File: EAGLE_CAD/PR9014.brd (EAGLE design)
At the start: 68.1 x 70.2 mm, 69 parts, among them J1 M3_SCREW_POST, SW1 C&K_PTS645

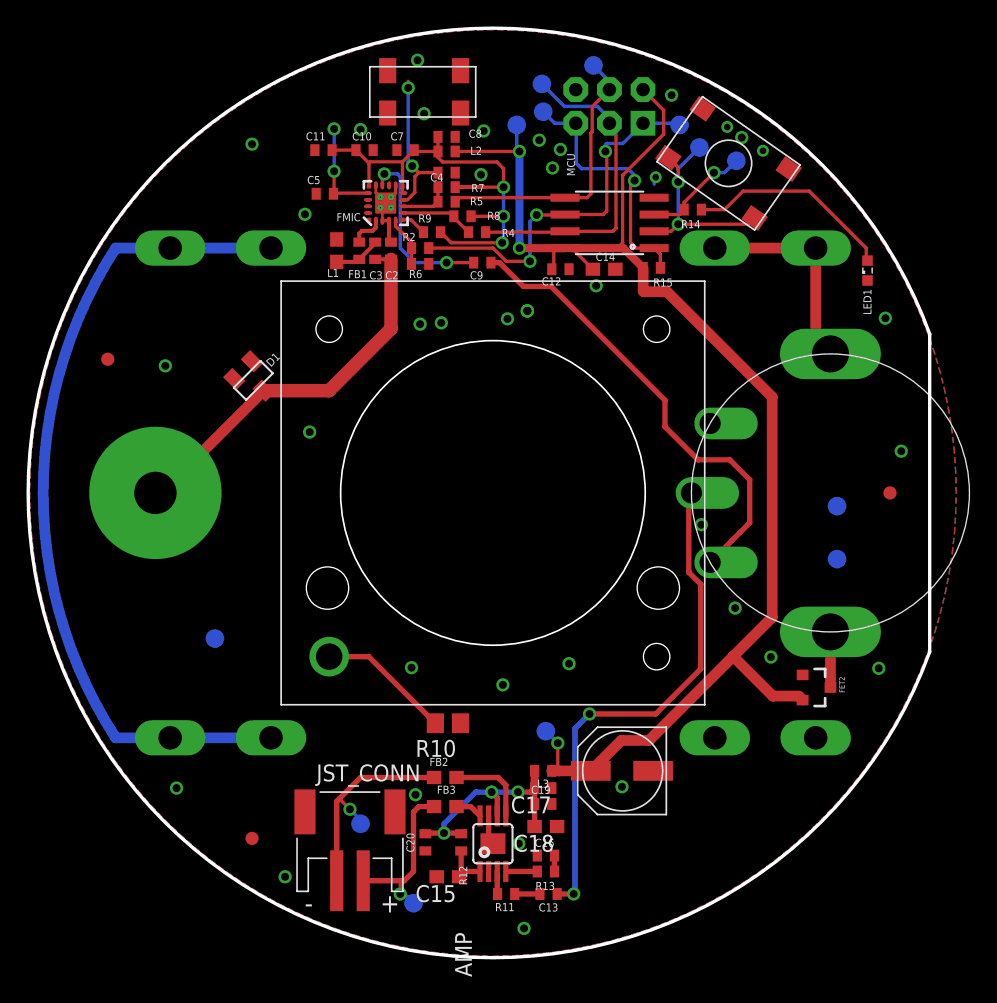
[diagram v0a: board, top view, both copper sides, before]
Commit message: bunch of routing stuff
and made the test points larger

pretty close to being released for this round
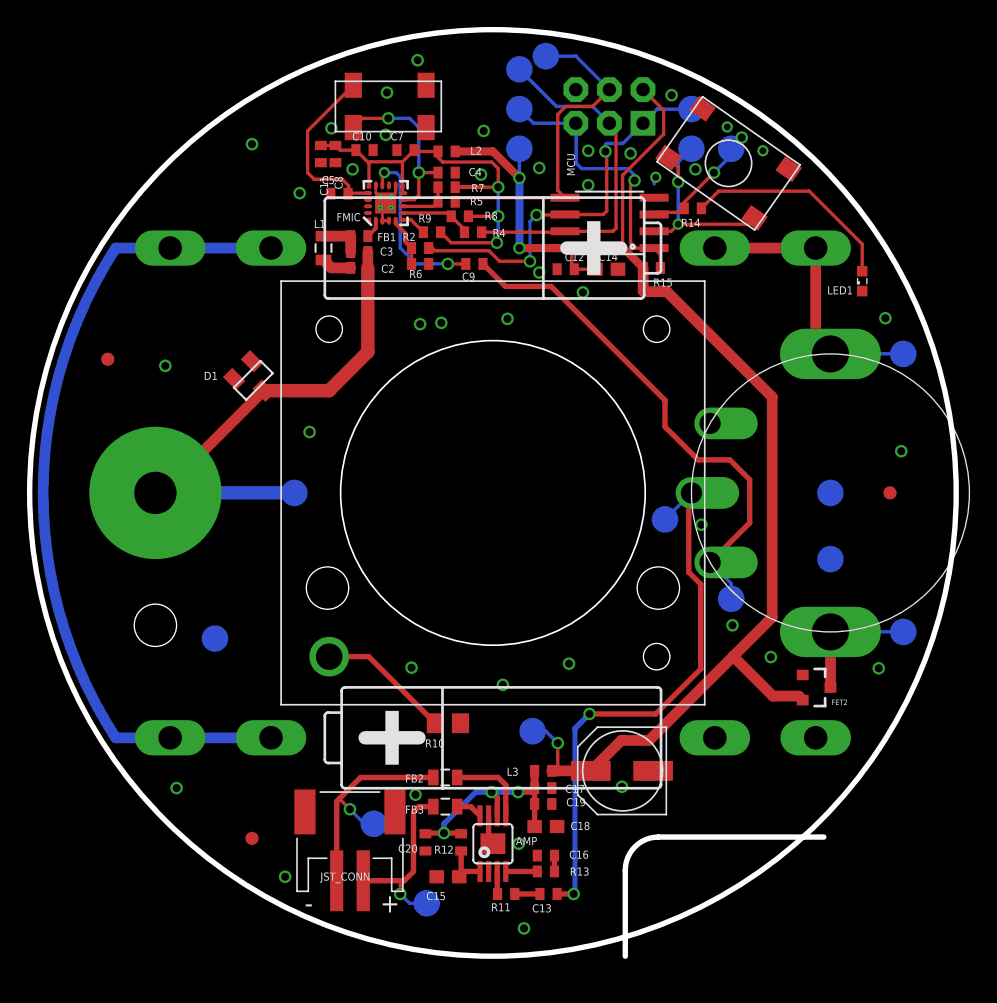
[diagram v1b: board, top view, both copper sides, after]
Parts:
- added TP14, TP15, TP16, TP17, TP18: TPTP20R, testpad:TP20R
- FB2, FB3, L1: device SparkFun-Passives:0603 -> SparkFun-Passives:0805
- TP1, TP10, TP11, TP12, TP13, TP2, TP3, TP4, TP5, TP6, TP7, TP8, TP9: value TPTP14R -> TPTP20R; device testpad:TP14R -> testpad:TP20R
- moved C8 8.50 mm to (23.1, 60.6), turned to 270 degrees
- moved TP13 3.67 mm to (39.0, 68.0)
- moved U$6 2.82 mm to (27.2, 64.2)
- moved C2 2.73 mm to (24.9, 52.0), turned to 180 degrees
- moved TP11 2.02 mm to (37.0, 67.0)
- moved TP12 1.81 mm to (37.0, 64.0)
- moved TP5 1.81 mm to (37.0, 61.0)
- moved TP10 1.50 mm to (50.0, 64.0)
- moved C3 1.20 mm to (24.9, 53.2), turned to 180 degrees
- moved TP2 1.12 mm to (60.5, 35.0)
- moved FB1 1.10 mm to (24.9, 54.4), turned to 0 degrees
- moved C5 1.10 mm to (23.4, 57.6)
- moved L1 1.02 mm to (22.2, 53.5), turned to 270 degrees
- moved TP4 1.00 mm to (38.0, 17.0)
- moved TP6 1.00 mm to (26.0, 10.0)
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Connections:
- removed net N$14: C2.1, C3.1, D1.3, J1.P$1
- removed net N$15: JP5.POS, JP5.POS@2, R1.SW_OUT
- removed net N$2: C5.1, FMIC.17, U$6.P$1
- removed net N$34: FET2.3, R1.SW_IN
- new net ANT: C2.1, C3.1, D1.3, J1.P$1, TP18.TP
- new net N$10: C5.1, FMIC.17, U$6.P$4
- new net SW_IN: FET2.3, R1.SW_IN, TP14.TP
- new net SW_OUT: JP5.POS, JP5.POS@2, R1.SW_OUT, TP15.TP
- net A_IN: now also TP16.TP
- net A_OUT: now also TP17.TP
- net N$1: now also U$6.P$1; no longer U$6.P$4
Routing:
- net ANT: track 0.00 -> 38.5 mm
- net N$14: track 29.4 -> 0.00 mm
- net SW_OUT: track 0.00 -> 21.6 mm
- net N$15: track 16.1 -> 0.00 mm
- net N$10: track 0.00 -> 13.6 mm
- net SW_IN: track 0.00 -> 9.70 mm
- net N$2: track 7.49 -> 0.00 mm, vias 2 -> 0
- net N$34: track 4.20 -> 0.00 mm
- net SDIO: track 21.3 -> 25.5 mm
- net A_IN: track 35.0 -> 39.0 mm
- net A_OUT: track 38.9 -> 41.7 mm
- net SCLK: track 24.7 -> 26.9 mm
- net N$1: track 11.4 -> 13.4 mm
- net RESET: track 19.5 -> 21.4 mm
- net 3.3V: track 38.8 -> 37.3 mm
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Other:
- board size 68.1 x 70.2 mm -> 70 x 70 mm
